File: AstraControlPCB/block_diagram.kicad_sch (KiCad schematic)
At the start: 0 parts

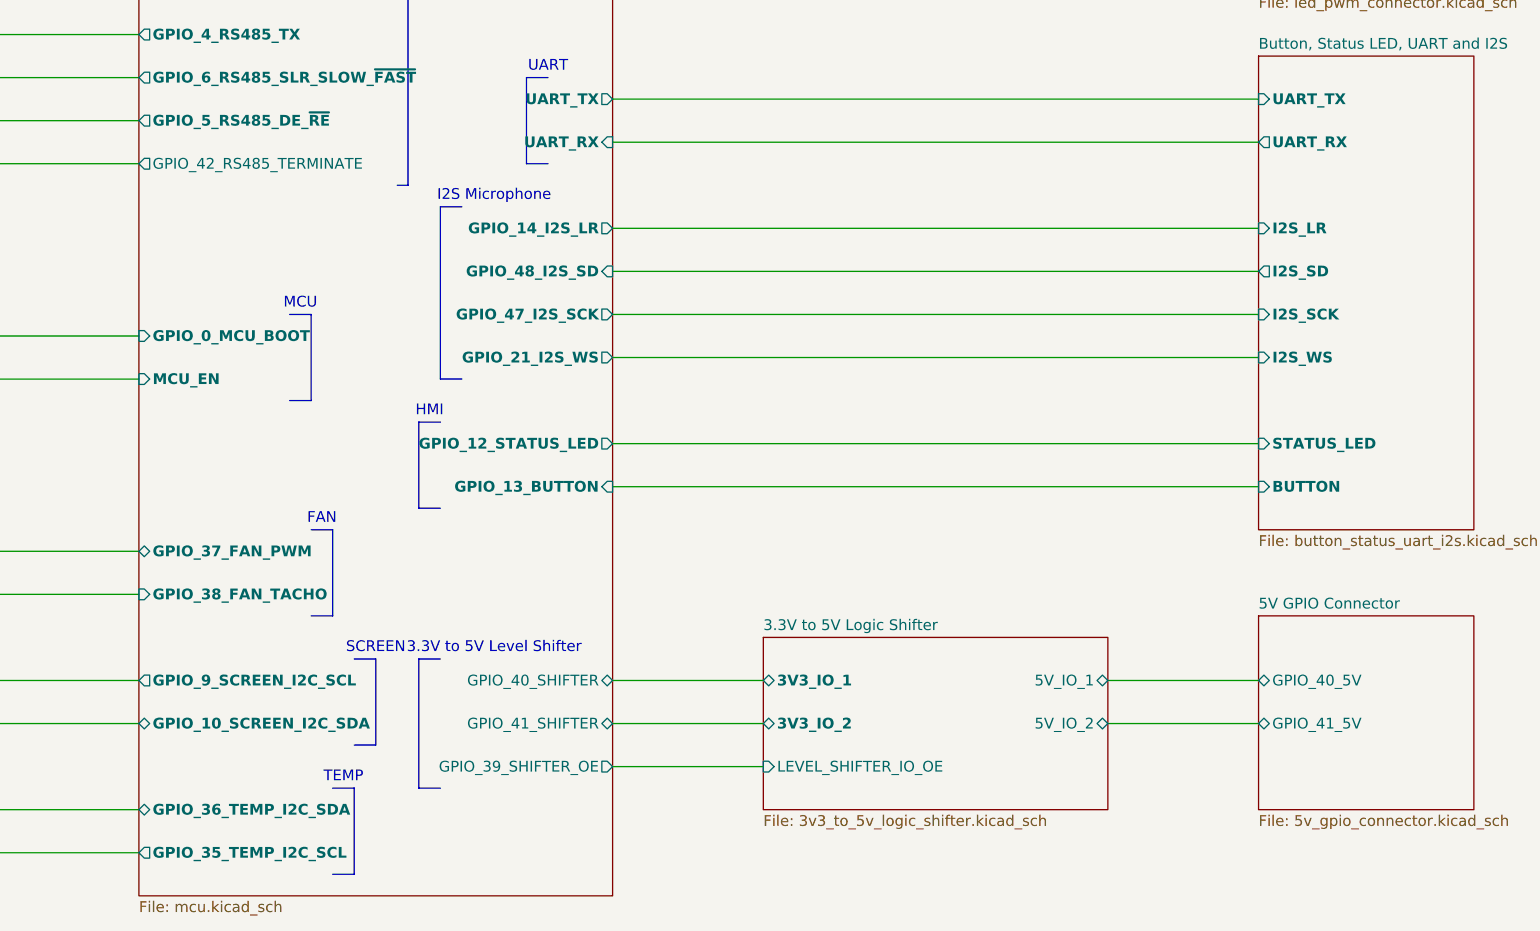
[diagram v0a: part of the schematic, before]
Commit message: Cleanup
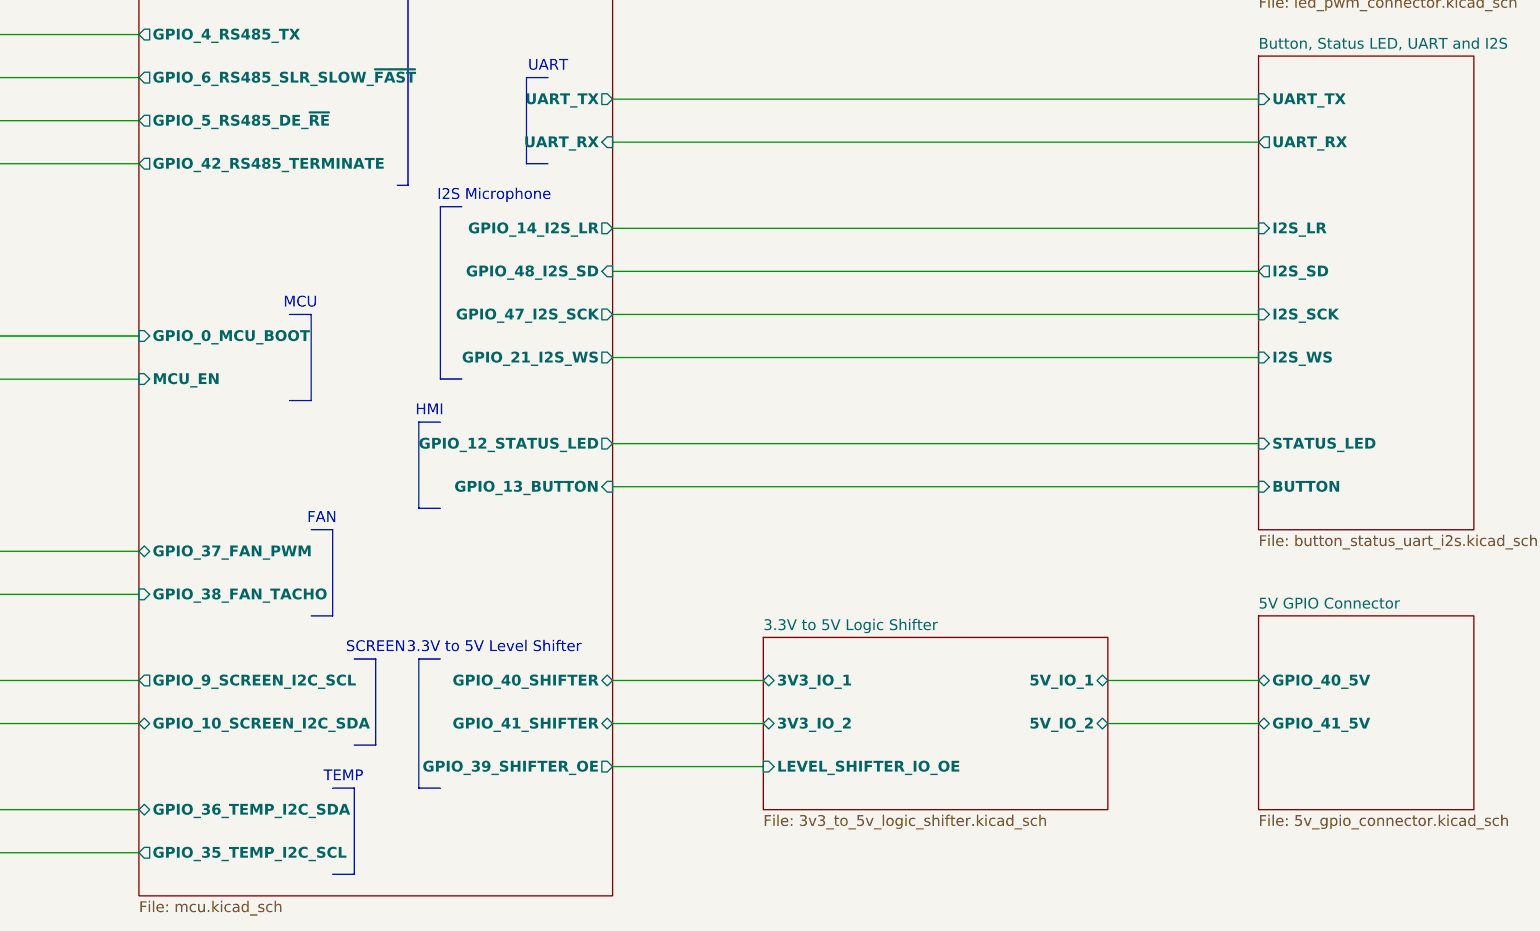
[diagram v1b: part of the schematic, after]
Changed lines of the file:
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@@
 				(font
 					(size 1.27 1.27)
+					(thickness 0.254)
+					(bold yes)
 				)
 				(justify right)
@@
 				(font
 					(size 1.27 1.27)
+					(thickness 0.254)
+					(bold yes)
 				)
 				(justify right)
@@
 				(font
 					(size 1.27 1.27)
+					(thickness 0.254)
+					(bold yes)
 				)
 				(justify left)
@@
 				(font
 					(size 1.27 1.27)
+					(thickness 0.254)
+					(bold yes)
 				)
 				(justify right)
@@
 				(font
 					(size 1.27 1.27)
+					(thickness 0.254)
+					(bold yes)
 				)
 				(justify left)
@@
 				(font
 					(size 1.27 1.27)
-				)
-				(justify left)
-			)
-		)
-		(instances
-			(project "AstraControl"
-				(path "/9a751838-dce8-4d69-8a02-736625ac74e7/0db21d8e-3390-4d67-877f-0e5d98e37848"
-					(page "16")
+					(thickness 0.254)
+					(bold yes)
+				)
+				(justify left)
+			)
+		)
+		(instances
+			(project "AstraControl"
+				(path "/9a751838-dce8-4d69-8a02-736625ac74e7/0db21d8e-3390-4d67-877f-0e5d98e37848"
+					(page "14")
 				)
 			)
@@
 			(project "AstraControl"
 				(path "/9a751838-dce8-4d69-8a02-736625ac74e7/0db21d8e-3390-4d67-877f-0e5d98e37848"
-					(page "13")
+					(page "11")
 				)
 			)
@@
 				(font
 					(size 1.27 1.27)
+					(thickness 0.254)
+					(bold yes)
 				)
 				(justify right)
@@
 				(font
 					(size 1.27 1.27)
+					(thickness 0.254)
+					(bold yes)
 				)
 				(justify right)
@@
 				(font
 					(size 1.27 1.27)
-				)
-				(justify left)
-			)
-		)
-		(instances
-			(project "AstraControl"
-				(path "/9a751838-dce8-4d69-8a02-736625ac74e7/0db21d8e-3390-4d67-877f-0e5d98e37848"
-					(page "15")
+					(thickness 0.254)
+					(bold yes)
+				)
+				(justify left)
+			)
+		)
+		(instances
+			(project "AstraControl"
+				(path "/9a751838-dce8-4d69-8a02-736625ac74e7/0db21d8e-3390-4d67-877f-0e5d98e37848"
+					(page "13")
 				)
 			)
@@
 			(project "AstraControl"
 				(path "/9a751838-dce8-4d69-8a02-736625ac74e7/0db21d8e-3390-4d67-877f-0e5d98e37848"
-					(page "14")
-				)
-			)
+					(page "12")
+				)
+			)
